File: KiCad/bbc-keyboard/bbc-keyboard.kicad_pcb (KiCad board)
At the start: 2 copper layers, 337.8 x 137.2 mm, 101 parts, among them IC1 74LS161, IC2 74251, IC3 74145, IC4 74LS30, SW1 escape, SW10 W, SW11 2, SW12 A, SW13 S, SW14 Z, SW15 f2, SW16 4, SW17 E, SW18 D, SW19 X, SW2 Q, SW20 C, SW21 space, SW22 f3, SW23 5, SW24 T, SW25 R, SW26 F, SW27 G, SW28 V, SW29 f5, SW3 F0, SW30 F4, SW31 7, SW32 6, SW33 Y, SW34 H, SW35 B, SW36 f6, SW37 8, SW38 9, SW39 U, SW4 1, SW40 J, SW41 N, SW42 M, SW43 f8, SW44 f7, SW45 I, SW46 O, SW47 K, SW48 L, SW49 <,, SW5 caps lk, SW50 f9, SW51 =-, SW52 0, SW53 P, SW54 @, SW55 ;+, SW56 >., SW57 \|, SW58 ~^, SW59 _£, SW6 shift lk, SW60 {[, SW61 *:, SW62 }], SW63 ?/, SW64 right, SW65 left, SW66 down, SW67 up, SW68 return, SW69 delete, SW7 tab, SW70 copy, SW71 shift, SW72 shift, SW73 ctrl, SW74 SW_DIP_x08, SW75 break, SW8 f1, SW9 3

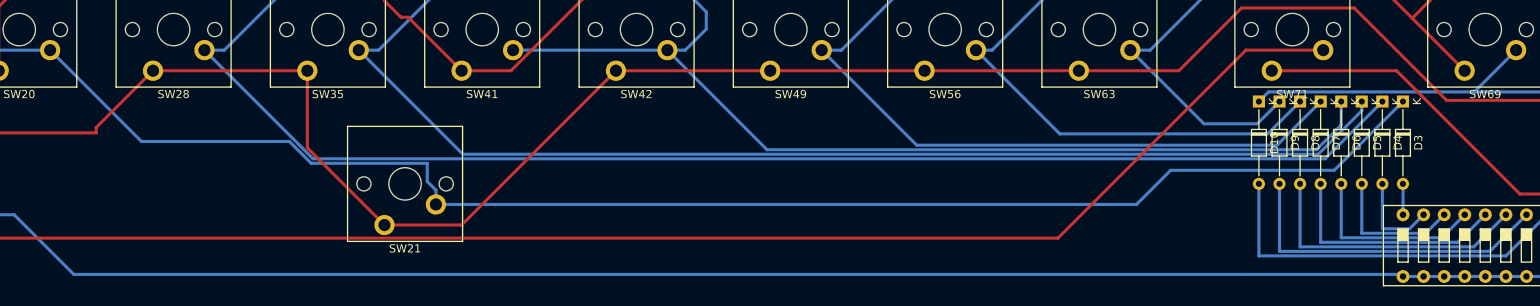
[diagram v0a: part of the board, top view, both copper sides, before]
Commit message: more layout tidying
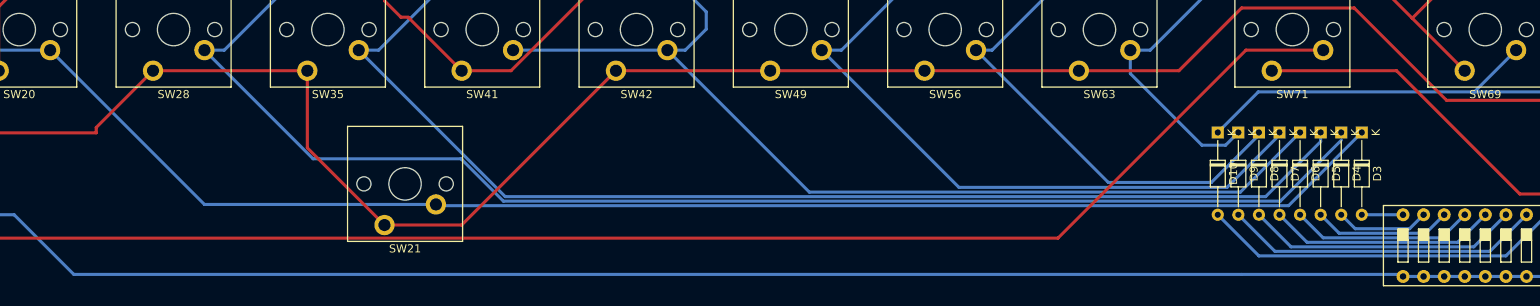
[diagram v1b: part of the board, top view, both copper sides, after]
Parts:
- moved D3 6.35 mm to (322.9, 209.6)
- moved D6 6.35 mm to (315.3, 209.6)
- moved D10 6.35 mm to (305.1, 209.6)
- moved D4 6.35 mm to (320.4, 209.6)
- moved D5 6.35 mm to (317.8, 209.6)
- moved D7 6.35 mm to (312.7, 209.6)
- moved D8 6.35 mm to (310.2, 209.6)
- moved D9 6.35 mm to (307.7, 209.6)
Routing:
- net /Key Matrix/KC_COL2: track 472.7 -> 463.8 mm
- net /Key Matrix/KC_COL9: track 221.6 -> 228.2 mm
- net /Key Matrix/KC_COL5: track 345.4 -> 341.4 mm
- net /Key Matrix/KC_COL8: track 207.2 -> 204.4 mm
- net /Key Matrix/KC_COL3: track 453.8 -> 451.1 mm
- net /Key Matrix/KC_COL4: track 391.7 -> 389.3 mm
- net /Key Matrix/KC_COL6: track 297.3 -> 295.1 mm
- net Net-(D10-Pad2): track 46.6 -> 44.9 mm
- net /Key Matrix/KC_COL7: track 250.3 -> 248.8 mm
- net Net-(D9-Pad2): track 40.7 -> 39.3 mm
- net Net-(D3-Pad2): track 3.81 -> 5.09 mm
- net Net-(D8-Pad2): track 34.8 -> 33.8 mm
- net Net-(D7-Pad2): track 29.0 -> 28.2 mm
